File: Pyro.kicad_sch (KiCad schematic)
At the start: 3 parts

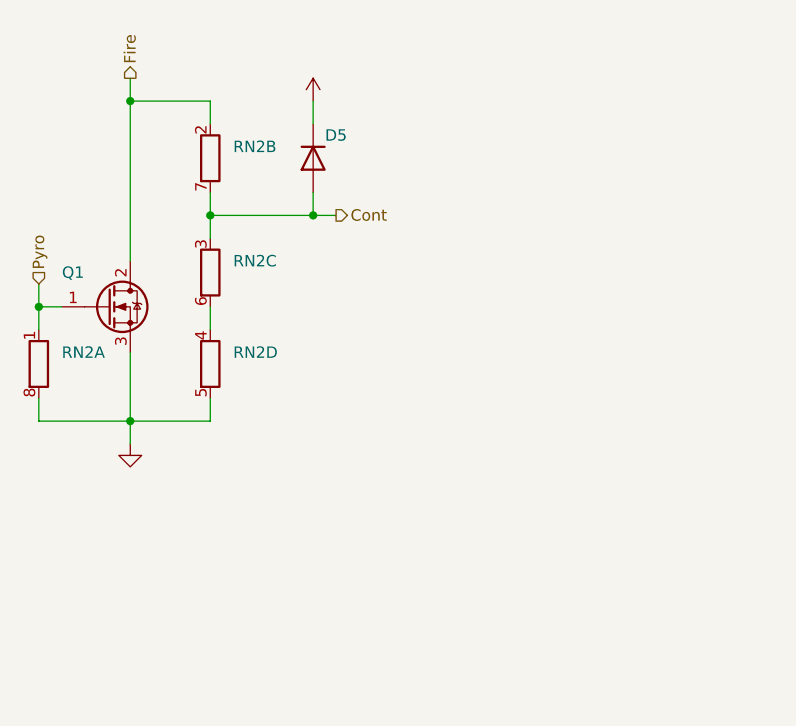
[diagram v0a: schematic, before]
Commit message: Rev 4 issued for production
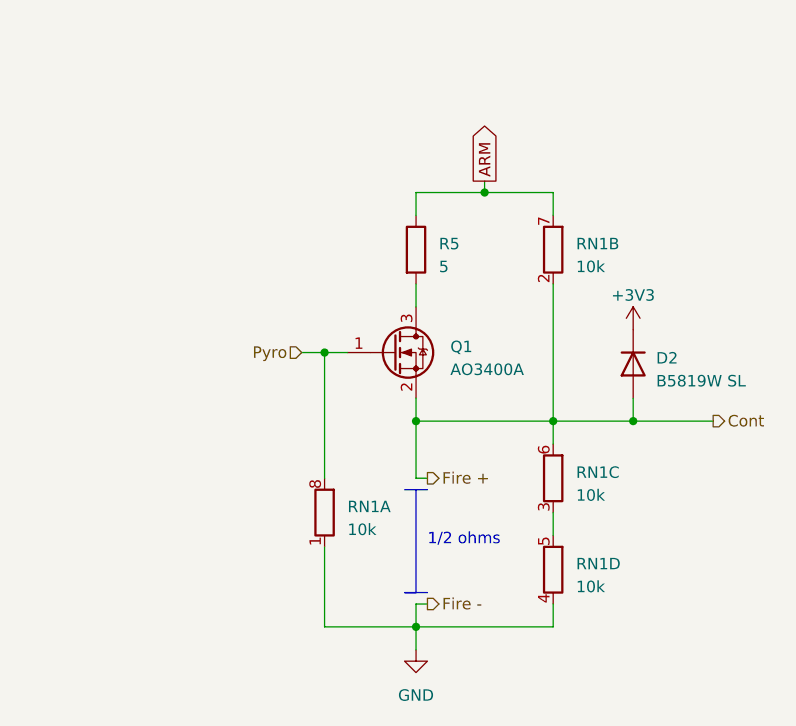
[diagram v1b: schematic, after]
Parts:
- removed D5: (no value), symbol Diode:1N914
- removed Q1: (no value), symbol Device:Q_NMOS_GDS
- removed RN2: (no value), Resistor_SMD:R_Array_Convex_4x0603, symbol Device:R_Pack04_Split
- added D2: B5819W SL, Diode_SMD:D_SOD-123, symbol Diode:1N914
- added Q1: AO3400A, Package_TO_SOT_SMD:SOT-23, symbol Transistor_FET:AO3400A
- added R5: 5, Resistor_SMD:R_0805_2012Metric, symbol Device:R
- added RN1: 10k, Resistor_SMD:R_Array_Convex_4x0603, symbol Device:R_Pack04_Split
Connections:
- net +3V3: now also D2.1 (K)
- net Cont: now also D2.2 (A), Q1.2 (S), RN1.2 (R2.1), RN1.6 (R3.2)
- net GND: now also RN1.1 (R1.1), RN1.4 (R4.1)
- net Pyro: now also Q1.1 (G), RN1.8 (R1.2)
- new net: Q1.3 (D), R5.2
- new net: RN1.3 (R3.1), RN1.5 (R4.2)
- new net ARM: R5.1, RN1.7 (R2.2)
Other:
- note added: "1/2 ohms"
- title: (none) -> Pyro Channel
